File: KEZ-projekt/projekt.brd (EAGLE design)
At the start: 68.9 x 86 mm, 42 parts, among them IC1 27C64P, IC2 4511N, IC3 4060N, IC4 4051N, IC5 4040N, IC6 U664N, T1 BC557, T2 BC557, T3 BC557, T4 BC557, T5 BC547, T6 BC547

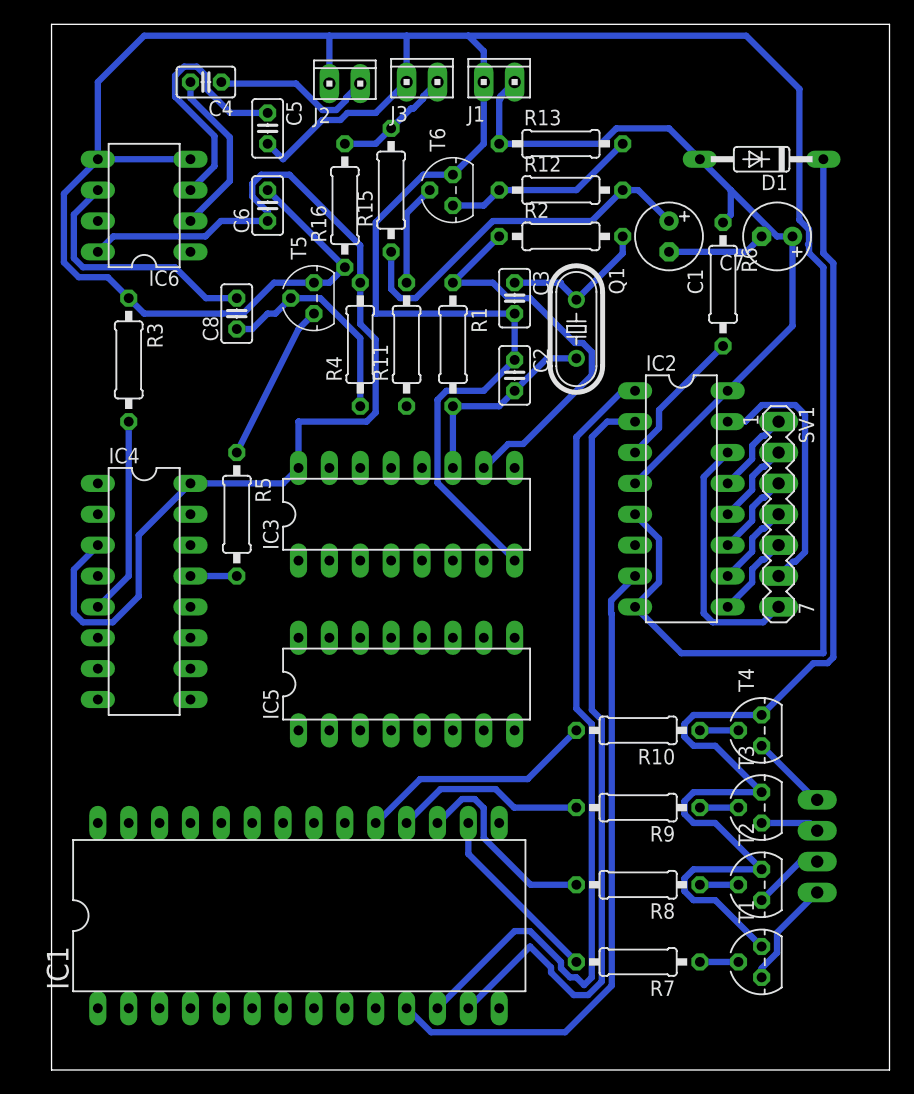
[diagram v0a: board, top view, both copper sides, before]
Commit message: completed - class 4
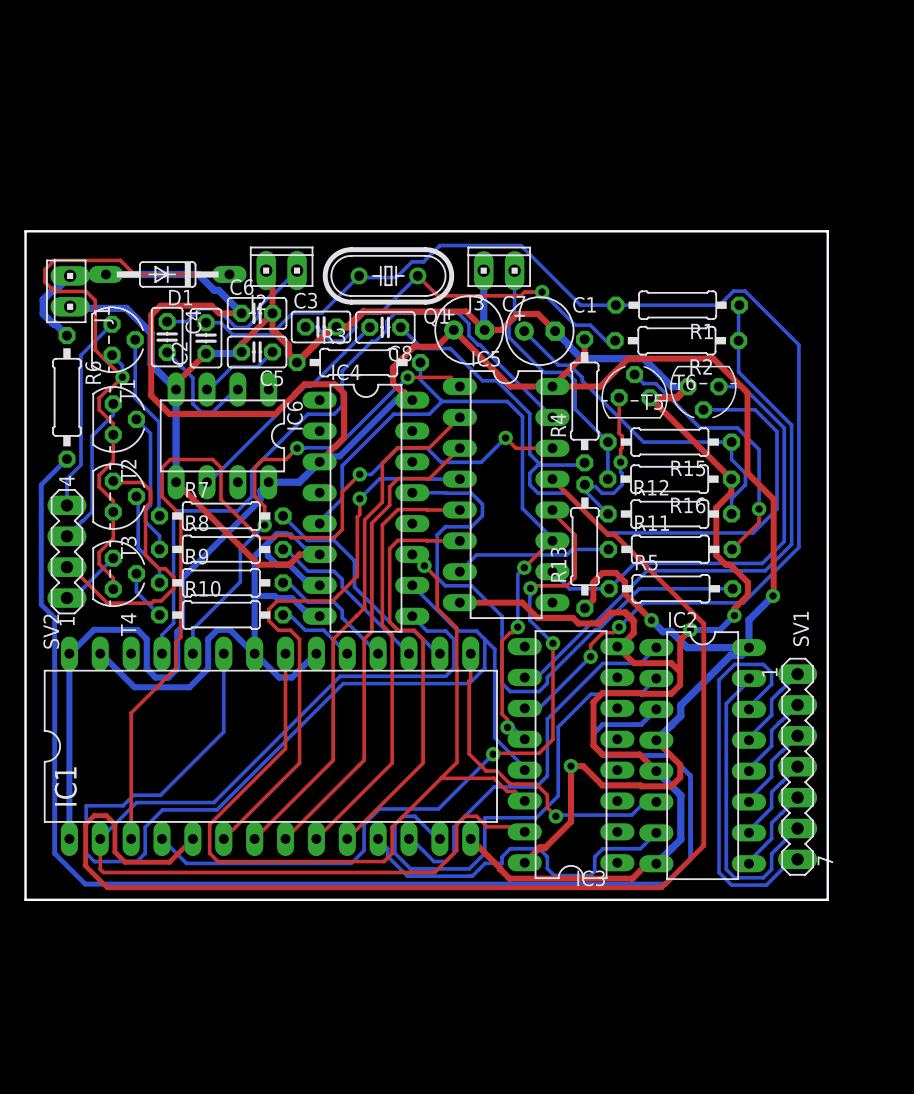
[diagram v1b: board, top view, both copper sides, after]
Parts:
- moved T1 74.0 mm to (45.6, 60.1), turned to 270 degrees
- moved SV2 66.3 mm to (41.9, 42.6), flipped to the top, turned to 90 degrees
- moved T2 65.7 mm to (45.7, 53.5), turned to 270 degrees
- moved T3 59.2 mm to (45.7, 47.2), turned to 270 degrees
- moved T4 54.9 mm to (45.7, 40.8), turned to 270 degrees
- moved R6 54.8 mm to (41.9, 55.3)
- moved R7 50.2 mm to (54.6, 45.6), turned to 0 degrees
- moved D1 49.8 mm to (50.2, 65.5)
- moved R8 44.0 mm to (54.6, 42.8), turned to 0 degrees
- moved J1 39.3 mm to (42.2, 64.1), turned to 90 degrees
- moved R9 39.0 mm to (54.6, 40.1), turned to 0 degrees
- moved R5 36.2 mm to (91.6, 39.6), turned to 0 degrees
- moved R10 35.6 mm to (54.6, 37.4), turned to 0 degrees
- moved R16 34.9 mm to (91.5, 48.6), turned to 180 degrees
- moved R13 33.2 mm to (84.5, 43.1), turned to 90 degrees
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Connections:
- removed net N$15: C7.+, D1.A, IC2.16, IC2.4, J1.1, R13.1, R6.1
- removed net N$16: C1.-, C7.-
- net GND: now also C1.-, C7.-
- net VCC: now also C7.+, D1.A, IC2.16, IC2.4, J1.1, R13.1, R6.1
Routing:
- net VCC: track 88.4 -> 241.9 mm, vias 0 -> 3
- net Q8: track 0.00 -> 104.9 mm
- net N$30: track 11.8 -> 110.7 mm
- net N$5: track 0.00 -> 87.4 mm
- net N$1: track 16.9 -> 102.0 mm, vias 0 -> 2
- net N$6: track 0.00 -> 82.7 mm
- net Q10: track 0.00 -> 76.2 mm, vias 0 -> 2
- net N$4: track 0.00 -> 70.6 mm, vias 0 -> 1
- net N$15: track 62.6 -> 0.00 mm
- net Q9: track 0.00 -> 62.1 mm, vias 0 -> 3
- net Q11: track 0.00 -> 57.4 mm
- net Q7: track 0.00 -> 46.9 mm, vias 0 -> 1
- net N$62: track 3.81 -> 50.2 mm
- net N$41: track 97.0 -> 51.9 mm, vias 0 -> 1
- net Q6: track 0.00 -> 43.2 mm
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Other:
- board size 68.9 x 86 mm -> 66 x 55 mm
